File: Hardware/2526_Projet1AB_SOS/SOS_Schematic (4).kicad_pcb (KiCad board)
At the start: 4 copper layers, 64 x 64 mm, 45 parts, among them J1 USB_B_Mini, J2 Conn_02x10_Odd_Even, J3 Conn_01x02, SW1 SW_SPDT, U1 BU33SD5WG-TR, U2 STM32L476RGTx, U3 HTRC11001T, U4 USBLC6-2SC6, Y1 13,56MHz, Y2 8MHz

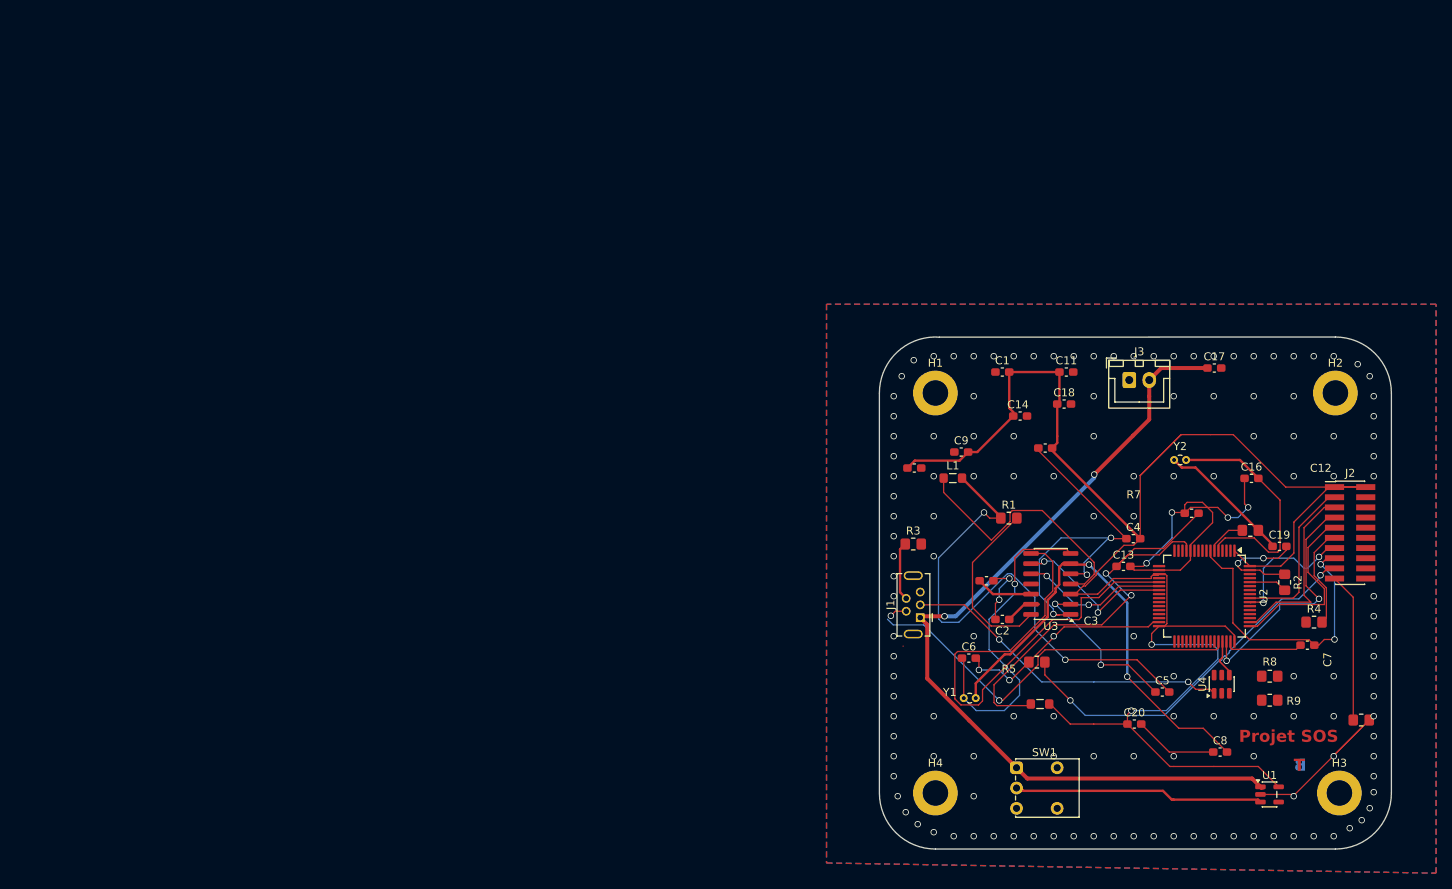
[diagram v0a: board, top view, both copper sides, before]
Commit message: schematic v2
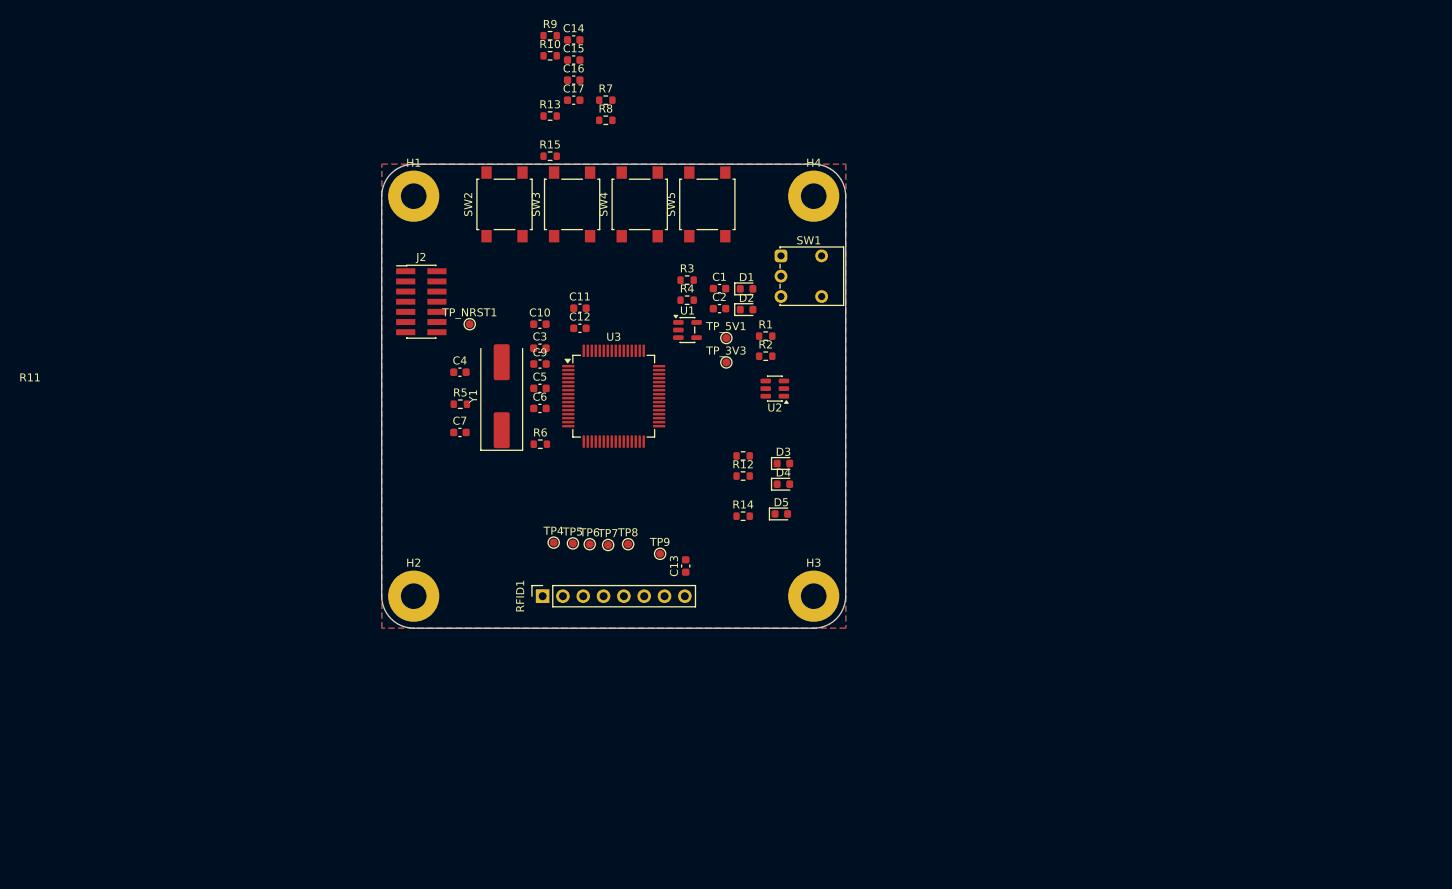
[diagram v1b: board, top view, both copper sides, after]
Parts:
- removed C18, C20: 1u, Capacitor_SMD:C_0603_1608Metric_Pad1.08x0.95mm_HandSolder
- removed C19: 20p, Capacitor_SMD:C_0603_1608Metric_Pad1.08x0.95mm_HandSolder
- removed C8: 22p, Capacitor_SMD:C_0603_1608Metric_Pad1.08x0.95mm_HandSolder
- removed J1: USB_B_Mini, Connector_USB:USB_Mini-B_Tensility_54-00023_Vertical
- removed J3: Conn_01x02, Connector_JST:JST_XH_B2B-XH-A_1x02_P2.50mm_Vertical
- removed L1: 1/2 uH, Inductor_SMD:L_0805_2012Metric_Pad1.05x1.20mm_HandSolder
- removed L2: L_Small, Inductor_SMD:L_0805_2012Metric_Pad1.05x1.20mm_HandSolder
- removed U4: USBLC6-2SC6, Package_TO_SOT_SMD:SOT-23-6
- removed Y2: 8MHz, Crystal:Crystal_DS10_D1.0mm_L4.3mm_Vertical
- added D1: RED, LED_SMD:LED_0603_1608Metric, F.Cu at (91.6, 61.6)
- added D2: RED, LED_SMD:LED_0603_1608Metric, F.Cu at (91.6, 64.2)
- added D3: RED, LED_SMD:LED_0603_1608Metric, F.Cu at (96.2, 83.4)
- added D4: GREEN, LED_SMD:LED_0603_1608Metric, F.Cu at (96.2, 86.0)
- added D5: BLUE, LED_SMD:LED_0603_1608Metric, F.Cu at (96.0, 89.7)
- added R10: 10k, Resistor_SMD:R_0603_1608Metric, F.Cu at (67.0, 32.5)
- added R11: 1k6, Resistor_SMD:R_0603_1608Metric, F.Cu at (91.2, 82.5)
- added R12: 1k1, Resistor_SMD:R_0603_1608Metric, F.Cu at (91.2, 85.0)
- added R13: 10k, Resistor_SMD:R_0603_1608Metric, F.Cu at (67.0, 40.0)
- added R14: 670R, Resistor_SMD:R_0603_1608Metric, F.Cu at (91.2, 90.0)
- added R15: 10k, Resistor_SMD:R_0603_1608Metric, F.Cu at (67.0, 45.0)
- added RFID1: RC522, Connector_PinSocket_2.54mm:PinSocket_1x08_P2.54mm_Vertical, F.Cu at (66.1, 100.0)
- added SW2: SW_Push, Button_Switch_SMD:SW_SPST_B3S-1000, F.Cu at (61.4, 51.0)
- added SW3: SW_Push, Button_Switch_SMD:SW_SPST_B3S-1000, F.Cu at (69.8, 51.0)
- added SW4: SW_Push, Button_Switch_SMD:SW_SPST_B3S-1000, F.Cu at (78.2, 51.0)
- added SW5: SW_Push, Button_Switch_SMD:SW_SPST_B3S-1000, F.Cu at (86.7, 51.0)
- added TP4: TP_NSS, TestPoint:TestPoint_Pad_D1.0mm, F.Cu at (67.5, 93.3)
- added TP5: TP_SCK, TestPoint:TestPoint_Pad_D1.0mm, F.Cu at (69.9, 93.4)
- added TP6: TP_MOSI, TestPoint:TestPoint_Pad_D1.0mm, F.Cu at (72.0, 93.5)
- added TP7: TP_MISO, TestPoint:TestPoint_Pad_D1.0mm, F.Cu at (74.3, 93.6)
- added TP8: TP_IRQ, TestPoint:TestPoint_Pad_D1.0mm, F.Cu at (76.8, 93.5)
- added TP9: TP_RST, TestPoint:TestPoint_Pad_D1.0mm, F.Cu at (80.8, 94.7)
- added TP_3V3: TP_3V3, TestPoint:TestPoint_Pad_D1.0mm, F.Cu at (89.1, 70.8)
- added TP_5V1: TP_5V, TestPoint:TestPoint_Pad_D1.0mm, F.Cu at (89.1, 67.7)
- added TP_NRST1: TP_NRST, TestPoint:TestPoint_Pad_D1.0mm, F.Cu at (57.0, 66.0)
- C1, C11, C2: value 100n -> 1u; footprint Capacitor_SMD:C_0603_1608Metric_Pad1.08x0.95mm_HandSolder -> Capacitor_SMD:C_0603_1608Metric
- C10, C13, C15: footprint Capacitor_SMD:C_0603_1608Metric_Pad1.08x0.95mm_HandSolder -> Capacitor_SMD:C_0603_1608Metric
- C12: value 10n -> 100n; footprint Capacitor_SMD:C_0603_1608Metric_Pad1.08x0.95mm_HandSolder -> Capacitor_SMD:C_0603_1608Metric
- C14: value 100n -> 10n; footprint Capacitor_SMD:C_0603_1608Metric_Pad1.08x0.95mm_HandSolder -> Capacitor_SMD:C_0603_1608Metric
- C16: value 20p -> 10n; footprint Capacitor_SMD:C_0603_1608Metric_Pad1.08x0.95mm_HandSolder -> Capacitor_SMD:C_0603_1608Metric
- C17: value 1u -> 10n; footprint Capacitor_SMD:C_0603_1608Metric_Pad1.08x0.95mm_HandSolder -> Capacitor_SMD:C_0603_1608Metric
- C3: value 100n -> 4u7; footprint Capacitor_SMD:C_0603_1608Metric_Pad1.08x0.95mm_HandSolder -> Capacitor_SMD:C_0603_1608Metric
- C4: value 10u -> 20p; footprint Capacitor_SMD:C_0603_1608Metric_Pad1.08x0.95mm_HandSolder -> Capacitor_SMD:C_0603_1608Metric
- C5: value 1,5n -> 100n; footprint Capacitor_SMD:C_0603_1608Metric_Pad1.08x0.95mm_HandSolder -> Capacitor_SMD:C_0603_1608Metric
- C6: value 22p -> 100n; footprint Capacitor_SMD:C_0603_1608Metric_Pad1.08x0.95mm_HandSolder -> Capacitor_SMD:C_0603_1608Metric
- C7: value 100n -> 20p; footprint Capacitor_SMD:C_0603_1608Metric_Pad1.08x0.95mm_HandSolder -> Capacitor_SMD:C_0603_1608Metric
- C9: value 4,7u -> 100n; footprint Capacitor_SMD:C_0603_1608Metric_Pad1.08x0.95mm_HandSolder -> Capacitor_SMD:C_0603_1608Metric
- H1, H2, H3, H4: footprint MountingHole:MountingHole_3.2mm_M3_DIN965_Pad -> MountingHole:MountingHole_3.2mm_M3_Pad
- J2: value Conn_02x10_Odd_Even -> Conn_ST_STDC14; footprint Connector_PinHeader_1.27mm:PinHeader_2x10_P1.27mm_Vertical_SMD -> Connector_PinHeader_1.27mm:PinHeader_2x07_P1.27mm_Vertical_SMD
- R1: value 2,2k -> 5k1; footprint Resistor_SMD:R_0805_2012Metric_Pad1.20x1.40mm_HandSolder -> Resistor_SMD:R_0603_1608Metric
- R2: value 10k -> 5k1; footprint Resistor_SMD:R_0805_2012Metric_Pad1.20x1.40mm_HandSolder -> Resistor_SMD:R_0603_1608Metric
- R3: value 100K -> 3k3; footprint Resistor_SMD:R_0805_2012Metric_Pad1.20x1.40mm_HandSolder -> Resistor_SMD:R_0603_1608Metric
- R4: value 10k -> 1k6; footprint Resistor_SMD:R_0805_2012Metric_Pad1.20x1.40mm_HandSolder -> Resistor_SMD:R_0603_1608Metric
- R5: value 10k -> 390; footprint Resistor_SMD:R_0805_2012Metric_Pad1.20x1.40mm_HandSolder -> Resistor_SMD:R_0603_1608Metric
- R6: footprint Resistor_SMD:R_0805_2012Metric_Pad1.20x1.40mm_HandSolder -> Resistor_SMD:R_0603_1608Metric
- R7: value 390 -> 10k; footprint Resistor_SMD:R_0805_2012Metric_Pad1.20x1.40mm_HandSolder -> Resistor_SMD:R_0603_1608Metric
- R8, R9: value 5k1 -> 10k; footprint Resistor_SMD:R_0805_2012Metric_Pad1.20x1.40mm_HandSolder -> Resistor_SMD:R_0603_1608Metric
- U2: value STM32L476RGTx -> USBLC6-2SC6; footprint Package_QFP:LQFP-64_10x10mm_P0.5mm -> Package_TO_SOT_SMD:SOT-23-6
- U3: value HTRC11001T -> STM32L476RGTx; footprint Package_SO:SOIC-14_3.9x8.7mm_P1.27mm -> Package_QFP:LQFP-64_10x10mm_P0.5mm
- Y1: value 13,56MHz -> 20MHz; footprint Crystal:Crystal_DS10_D1.0mm_L4.3mm_Vertical -> Crystal:Crystal_SMD_HC49-SD
- moved R9 122.4 mm to (67.0, 29.9)
- moved J2 119.6 mm to (51.0, 63.2)
- moved H2 118.0 mm to (50.0, 100.0)
- moved C7 109.2 mm to (55.8, 79.5)
- moved R6 108.3 mm to (65.8, 81.0)
- moved R8 108.2 mm to (74.0, 40.5)
- moved C16 98.3 mm to (70.0, 35.5)
- moved R7 96.9 mm to (74.0, 38.0)
- moved U1 93.1 mm to (84.2, 66.7)
- moved R4 88.1 mm to (84.2, 63.0)
- moved C17 86.8 mm to (70.0, 38.0)
- moved C4 86.7 mm to (55.8, 72.0)
- moved C5 86.6 mm to (65.8, 74.0)
- moved C12 79.9 mm to (70.8, 66.5)
- moved R5 78.9 mm to (55.8, 76.0)
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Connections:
- C1 pad 1: GND -> +5V
- C1 pad 2: +3.3V -> GND
- C12 pad 2: +3.3VA -> +3.3V
- C13 pad 1: +3.3VA -> +3.3V
- C14 pad 1: +3.3V -> /USR_BTN_1
- C15 pad 1: GND -> NRST
- C15 pad 2: +3.3V -> GND
- C16 pad 1: GND -> /USR_BTN_2
- C16 pad 2: OSC_IN -> GND
- C17 pad 1: +5V -> /USR_BTN_3
- C2 pad 1: Net-(U3-QGND) -> +3.3V
- C3 pad 1: Net-(U3-CEXT) -> GND
- C3 pad 2: GND -> +3.3V
- C4 pad 2: +3.3V -> OSC_IN
- C5 pad 1: Net-(U3-TX2) -> +3.3V
- C5 pad 2: Net-(C5-Pad2) -> GND
- C6 pad 1: Net-(U3-XTAL2) -> +3.3V
- C7 pad 1: GND -> Net-(C7-Pad1)
- C7 pad 2: NRST -> GND
- C9 pad 1: GND -> +3.3V
- C9 pad 2: +3.3V -> GND
- J2 pad 1: +3.3V -> unconnected-(J2-NC-Pad1)
- J2 pad 10: GND -> unconnected-(J2-JTDI/NC-Pad10)
- J2 pad 11: Net-(J2-Pin_11) -> GND
- J2 pad 12: GND -> NRST
- J2 pad 13: TDO -> UART_RX
- J2 pad 14: GND -> UART_TX
- J2 pad 2: +3.3V -> unconnected-(J2-NC-Pad2)
- J2 pad 3: TRST -> +3.3V
- J2 pad 4: GND -> SWDIO
- J2 pad 5: TDI -> GND
- J2 pad 6: GND -> SWCLK
- J2 pad 7: SWDIO -> GND
- J2 pad 8: GND -> SWO
- J2 pad 9: SWDCK -> unconnected-(J2-JRCLK/NC-Pad9)
- R1 pad 1: Net-(C5-Pad2) -> Net-(J1-CC1)
- R1 pad 2: Net-(U3-RX) -> GND
- R2 pad 2: Net-(U2-BOOT0) -> Net-(J1-CC2)
- R3 pad 1: Net-(J1-ID) -> +5V
- R3 pad 2: GND -> Net-(D1-A)
- R4 pad 1: GND -> +3.3V
- R4 pad 2: Net-(J2-Pin_11) -> Net-(D2-A)
- R5 pad 1: GND -> OSC_OUT
- R5 pad 2: Net-(J2-Pin_17) -> Net-(C7-Pad1)
- R6 pad 1: Net-(J2-Pin_19) -> GND
- R6 pad 2: GND -> Net-(U3-BOOT0)
- R7 pad 1: OSC_OUT -> /USR_BTN_1
- R7 pad 2: Net-(C19-Pad1) -> Net-(R7-Pad2)
- R8 pad 1: Net-(J5-CC1) -> Net-(R7-Pad2)
- R9 pad 1: GND -> /USR_BTN_2
- U2 pad 1: +3.3V -> USBDP
- U2 pad 2: unconnected-(U2-PC13-Pad2) -> GND
- U2 pad 3: unconnected-(U2-PC14-Pad3) -> USBDM
- U2 pad 4: unconnected-(U2-PC15-Pad4) -> D+
- U2 pad 5: OSC_IN -> +5V
- U2 pad 6: OSC_OUT -> D-
- U3 pad 1: GND -> +3.3V
- U3 pad 10: SPI1_MISO -> unconnected-(U3-PC2-Pad10)
- U3 pad 11: (no net) -> unconnected-(U3-PC3-Pad11)
- U3 pad 12: Net-(U3-CEXT) -> GND
- U3 pad 13: Net-(U3-QGND) -> +3.3V
- U3 pad 14: Net-(U3-RX) -> unconnected-(U3-PA0-Pad14)
- U3 pad 2: Net-(U3-TX2) -> unconnected-(U3-PC13-Pad2)
- U3 pad 3: +3.3V -> unconnected-(U3-PC14-Pad3)
- U3 pad 4: Net-(U3-TX1) -> unconnected-(U3-PC15-Pad4)
- U3 pad 5: GND -> OSC_IN
- U3 pad 6: Net-(U3-XTAL1) -> OSC_OUT
- U3 pad 7: Net-(U3-XTAL2) -> NRST
- U3 pad 8: SPI1_SCK -> unconnected-(U3-PC0-Pad8)
- U3 pad 9: SPI1_MOSI -> unconnected-(U3-PC1-Pad9)
- Y1 pad 1: Net-(U3-XTAL2) -> Net-(C7-Pad1)
- Y1 pad 2: Net-(U3-XTAL1) -> OSC_IN
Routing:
- net +3.3V: track 229.0 -> 0.00 mm, vias 2 -> 0
- net GND: track 186.6 -> 0.00 mm, vias 150 -> 0
- net +5V: track 107.4 -> 0.00 mm, vias 2 -> 0
- net Net-(C5-Pad2): track 65.1 -> 0.00 mm, vias 2 -> 0
- net SPI1_SCK: track 63.6 -> 0.00 mm
- net +3.3VA: track 58.9 -> 0.00 mm, vias 2 -> 0
- net Net-(U3-XTAL1): track 57.6 -> 0.00 mm, vias 2 -> 0
- net D-: track 49.7 -> 0.00 mm, vias 1 -> 0
- net Net-(J2-Pin_17): track 47.8 -> 0.00 mm, vias 2 -> 0
- net USBDP: track 41.3 -> 0.00 mm, vias 2 -> 0
- net Net-(U3-XTAL2): track 41.2 -> 0.00 mm, vias 1 -> 0
- net NRST: track 37.7 -> 0.00 mm, vias 2 -> 0
- net Net-(U3-TX1): track 32.9 -> 0.00 mm
- net SWDIO: track 31.4 -> 0.00 mm, vias 2 -> 0
- net Net-(SW1-B): track 31.2 -> 0.00 mm
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- added copper zone on In1.Cu, net +3.3V
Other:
- board size 64 x 64 mm -> 58 x 58 mm
- board text removed: "B"
- board text removed: "Projet SOS"
- board text removed: "T"

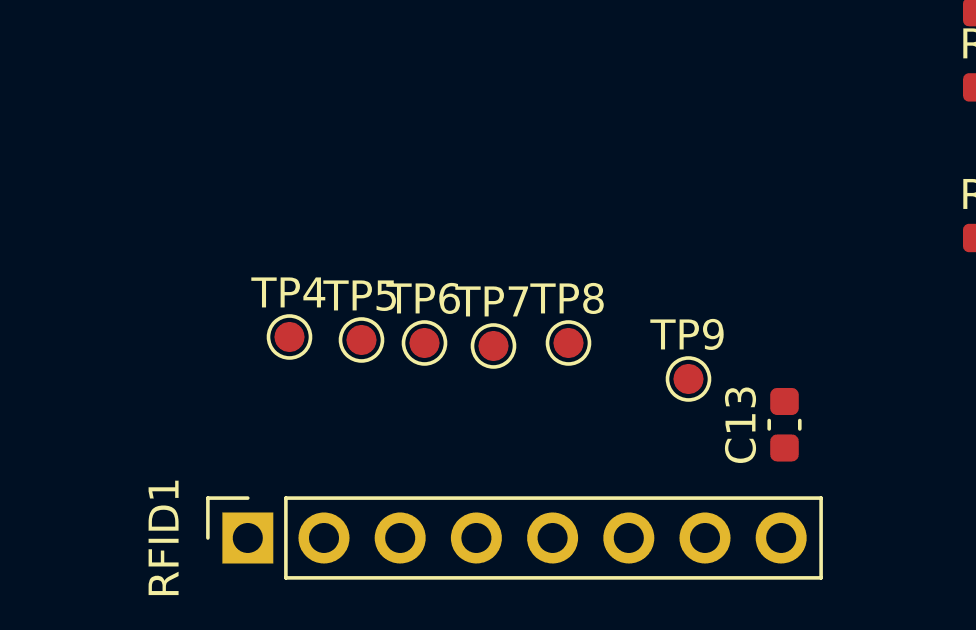
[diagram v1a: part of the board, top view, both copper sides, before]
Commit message: BOM
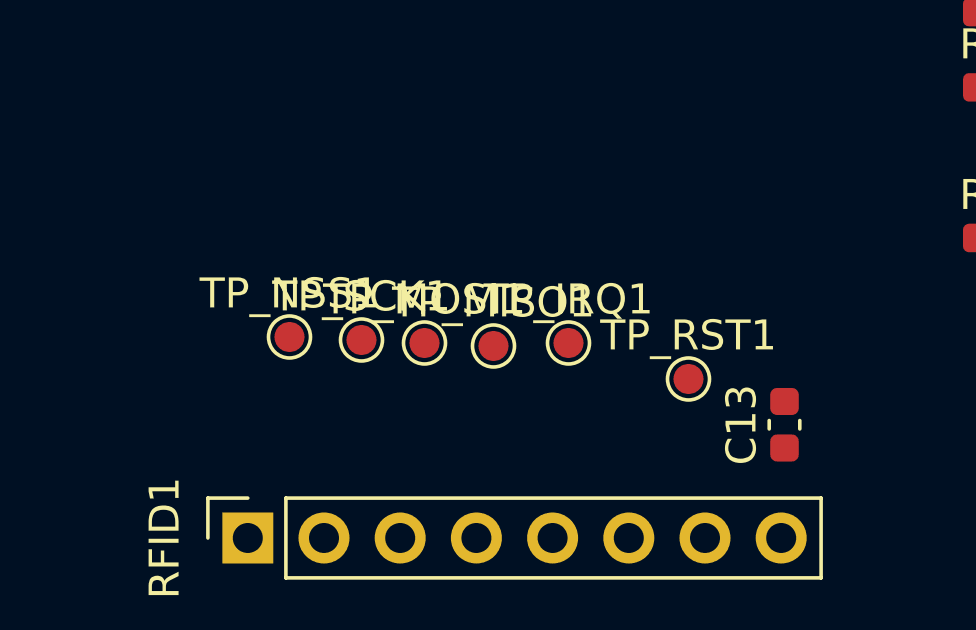
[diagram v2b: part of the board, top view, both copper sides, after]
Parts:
- TP_3V3: value TP_3V3 -> TestPoint
- TP_5V1: value TP_5V -> TestPoint
- TP_IRQ1: renamed from TP8; value TP_IRQ -> TestPoint
- TP_MISO1: renamed from TP7; value TP_MISO -> TestPoint
- TP_MOSI1: renamed from TP6; value TP_MOSI -> TestPoint
- TP_NRST1: value TP_NRST -> TestPoint
- TP_NSS1: renamed from TP4; value TP_NSS -> TestPoint
- TP_RST1: renamed from TP9; value TP_RST -> TestPoint
- TP_SCK1: renamed from TP5; value TP_SCK -> TestPoint
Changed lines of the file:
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@@
 		(descr "SMD pad as test Point, diameter 1.0mm")
 		(tags "test point SMD pad")
-		(property "Reference" "TP5"
+		(property "Reference" "TP_SCK1"
 			(at 0 -1.448 0)
 			(layer "F.SilkS")
@@
 			)
 		)
-		(property "Value" "TP_SCK"
+		(property "Value" "TestPoint"
 			(at 0 1.55 0)
 			(layer "F.Fab")
@@
 			)
 		)
-		(property "Value" "TP_5V"
+		(property "Value" "TestPoint"
 			(at 0 1.55 0)
 			(layer "F.Fab")
@@
 		(descr "SMD pad as test Point, diameter 1.0mm")
 		(tags "test point SMD pad")
-		(property "Reference" "TP9"
+		(property "Reference" "TP_RST1"
 			(at 0 -1.448 0)
 			(layer "F.SilkS")
@@
 			)
 		)
-		(property "Value" "TP_RST"
+		(property "Value" "TestPoint"
 			(at 0 1.55 0)
 			(layer "F.Fab")
@@
 		(descr "SMD pad as test Point, diameter 1.0mm")
 		(tags "test point SMD pad")
-		(property "Reference" "TP4"
+		(property "Reference" "TP_NSS1"
 			(at 0 -1.448 0)
 			(layer "F.SilkS")
@@
 			)
 		)
-		(property "Value" "TP_NSS"
+		(property "Value" "TestPoint"
 			(at 0 1.55 0)
 			(layer "F.Fab")
@@
 		(descr "SMD pad as test Point, diameter 1.0mm")
 		(tags "test point SMD pad")
-		(property "Reference" "TP7"
+		(property "Reference" "TP_MISO1"
 			(at 0 -1.448 0)
 			(layer "F.SilkS")
@@
 			)
 		)
-		(property "Value" "TP_MISO"
+		(property "Value" "TestPoint"
 			(at 0 1.55 0)
 			(layer "F.Fab")
@@
 			)
 		)
-		(property "Value" "TP_NRST"
+		(property "Value" "TestPoint"
 			(at 0 1.55 0)
 			(layer "F.Fab")
@@
 			)
 		)
-		(property "Value" "TP_3V3"
+		(property "Value" "TestPoint"
 			(at 0 1.55 0)
 			(layer "F.Fab")
@@
 		(descr "SMD pad as test Point, diameter 1.0mm")
 		(tags "test point SMD pad")
-		(property "Reference" "TP6"
+		(property "Reference" "TP_MOSI1"
 			(at 0 -1.448 0)
 			(layer "F.SilkS")
@@
 			)
 		)
-		(property "Value" "TP_MOSI"
+		(property "Value" "TestPoint"
 			(at 0 1.55 0)
 			(layer "F.Fab")
@@
 		(descr "SMD pad as test Point, diameter 1.0mm")
 		(tags "test point SMD pad")
-		(property "Reference" "TP8"
+		(property "Reference" "TP_IRQ1"
 			(at 0 -1.448 0)
 			(layer "F.SilkS")
@@
 			)
 		)
-		(property "Value" "TP_IRQ"
+		(property "Value" "TestPoint"
 			(at 0 1.55 0)
 			(layer "F.Fab")
